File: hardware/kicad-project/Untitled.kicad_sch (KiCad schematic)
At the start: 42 parts, among them CN2 ST-0322D00-071-1A2H, Q1 DMG2301L-7, Q2 DMG2301L-7, SW1 TS-1187A-B-A-B, SW2 TS-1187A-B-A-B, U1 ESP32-S3-WROOM-1-N8, U2 MCP73831-2ACI/MC, U4 XC6220B331MR, U6 MAX98357AETE+T

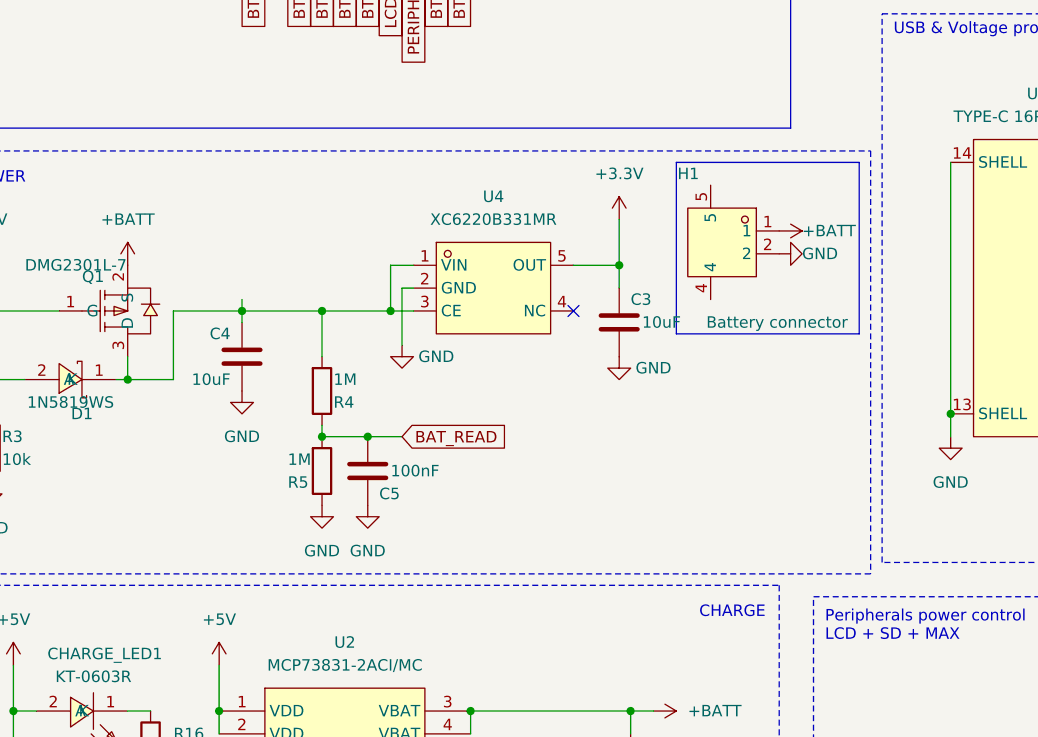
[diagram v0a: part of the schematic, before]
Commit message: wip
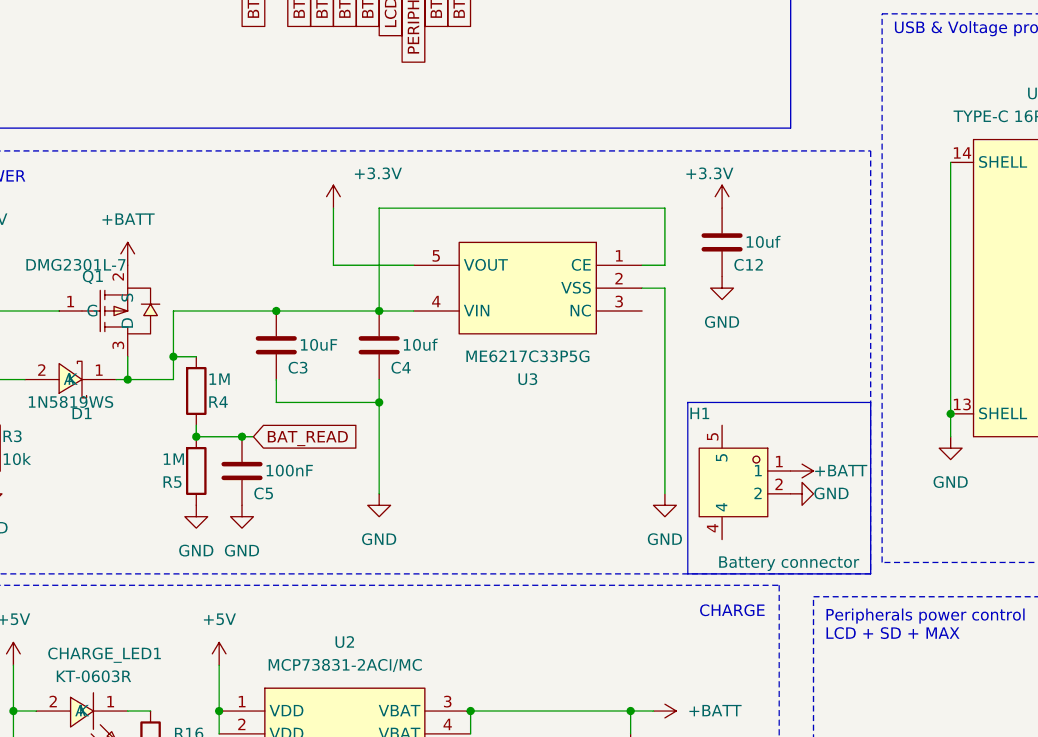
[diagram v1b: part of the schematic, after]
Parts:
- removed U4: XC6220B331MR, easyeda2kicad:SOT-23-5_L2.9-W1.6-P0.95-LS2.8-BR, symbol easyedaToKicad:XC6220B331MR
- added C12: 10uf, Capacitor_SMD:C_0603_1608Metric, symbol Device:C
- added U3: ME6217C33P5G, easyeda2kicad:SOT-89-5_L4.5-W2.5-P1.50-LS4.5-BR, symbol easyedaToKicad:ME6217C33P5G
- C4: value 10uF -> 10uf
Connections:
- net +3.3V: now also C12.2, U3.5 (VOUT); no longer C3.1
- net GND: now also C3.1, C12.1, U3.2 (VSS); no longer C3.2
- net at C4.2, D1.1 (K), Q1.3 (D)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: now also C3.2, U3.1 (CE), U3.4 (VIN)
- no-connect marks 7 -> 6
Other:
- moved on the sheet: C5, H1, R4, R5

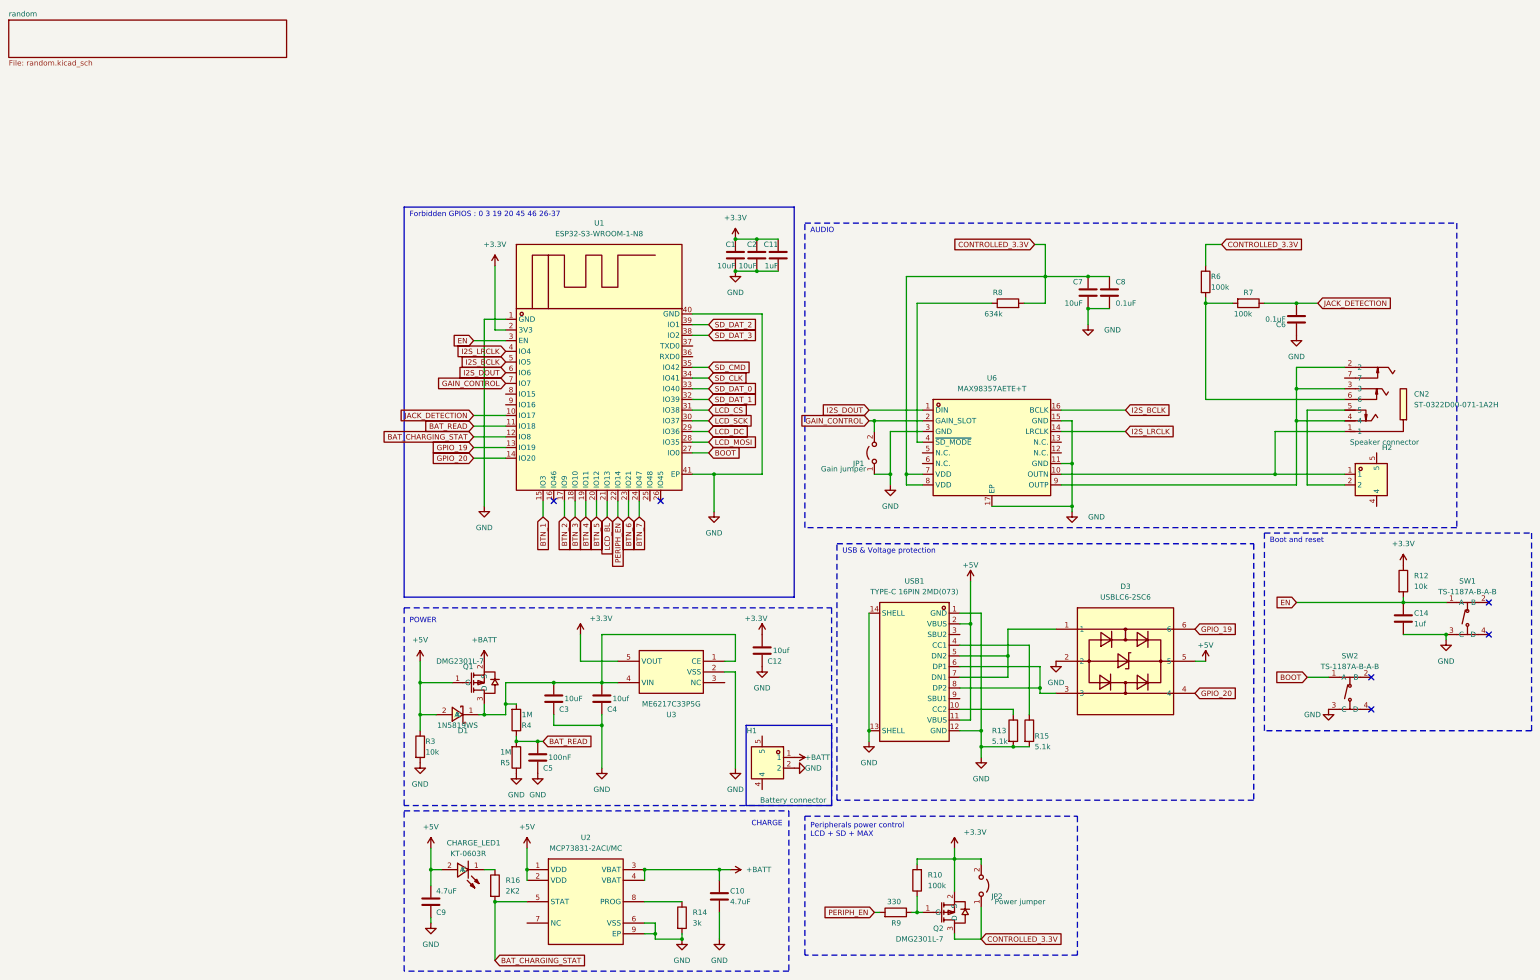
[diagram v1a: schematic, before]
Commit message: wip
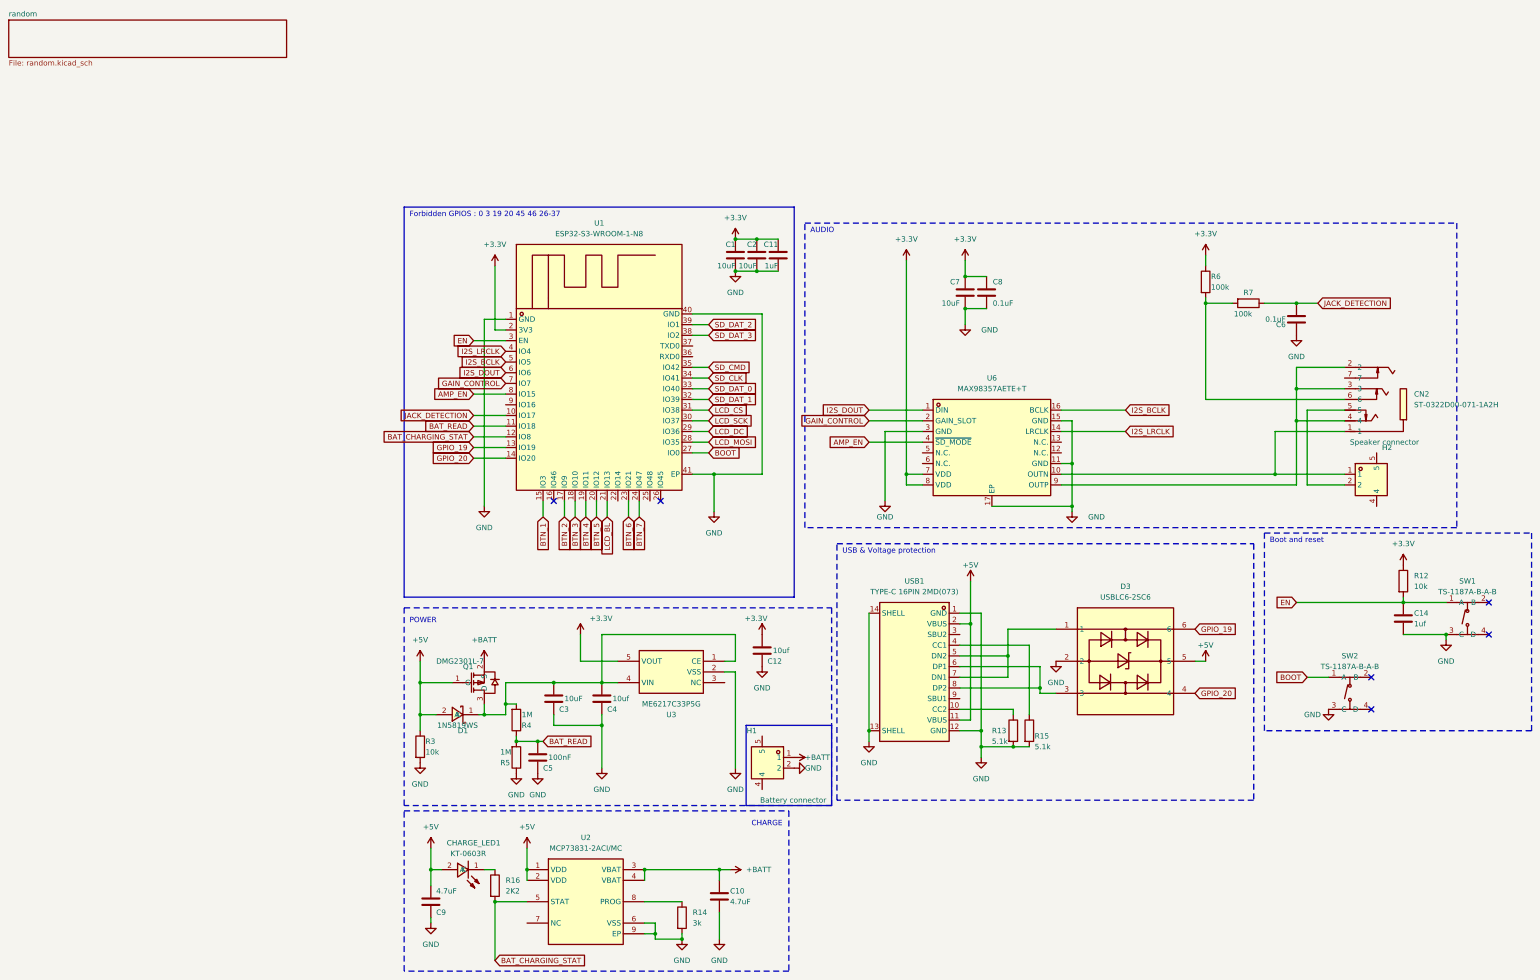
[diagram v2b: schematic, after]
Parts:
- removed JP1: Gain jumper, Jumper:SolderJumper-2_P1.3mm_Open_Pad1.0x1.5mm, symbol Jumper:Jumper_2_Open
- removed JP2: Power jumper, Jumper:SolderJumper-2_P1.3mm_Open_Pad1.0x1.5mm, symbol Jumper:Jumper_2_Open
- removed Q2: DMG2301L-7, easyeda2kicad:SOT-23-3_L2.9-W1.3-P1.90-LS2.4-BR, symbol easyedaToKicad:DMG2301L-7
- removed R10: 100k, Resistor_SMD:R_0603_1608Metric, symbol Device:R
- removed R8: 634k, Resistor_SMD:R_0603_1608Metric, symbol Device:R
- removed R9: 330, Resistor_SMD:R_0603_1608Metric, symbol Device:R
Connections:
- net CONTROLLED_3.3V is gone; now on net +3.3V: C7.2, C8.2, R6.1, U6.7 (VDD), U6.8 (VDD)
- net AMP_EN: now reaches U1.8 (IO15)
- net AMP_EN: now also U6.4 (~{SD_MODE})
- net PERIPH_EN: no longer names the net of U1.22 (IO14)
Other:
- note removed: "Peripherals power control LCD + SD + MAX"
- moved on the sheet: C7, C8
